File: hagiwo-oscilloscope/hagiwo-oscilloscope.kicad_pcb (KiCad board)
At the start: 2 copper layers, 40.2 x 111.8 mm, 25 parts, among them J1 Encoder Header, J2 10-Pin uZeus Power, J3 OLED Header, J4 Input Header, U1 Opamp_Dual

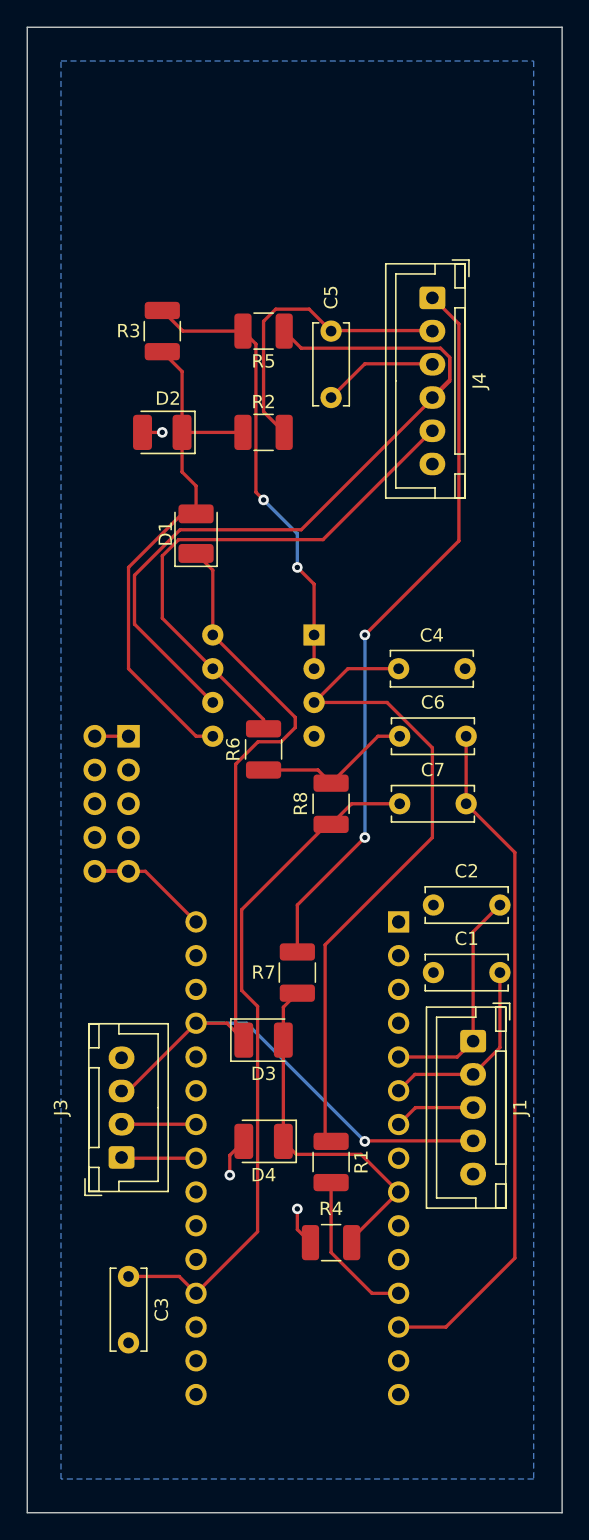
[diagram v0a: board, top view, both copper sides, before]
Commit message: o-scope rev2
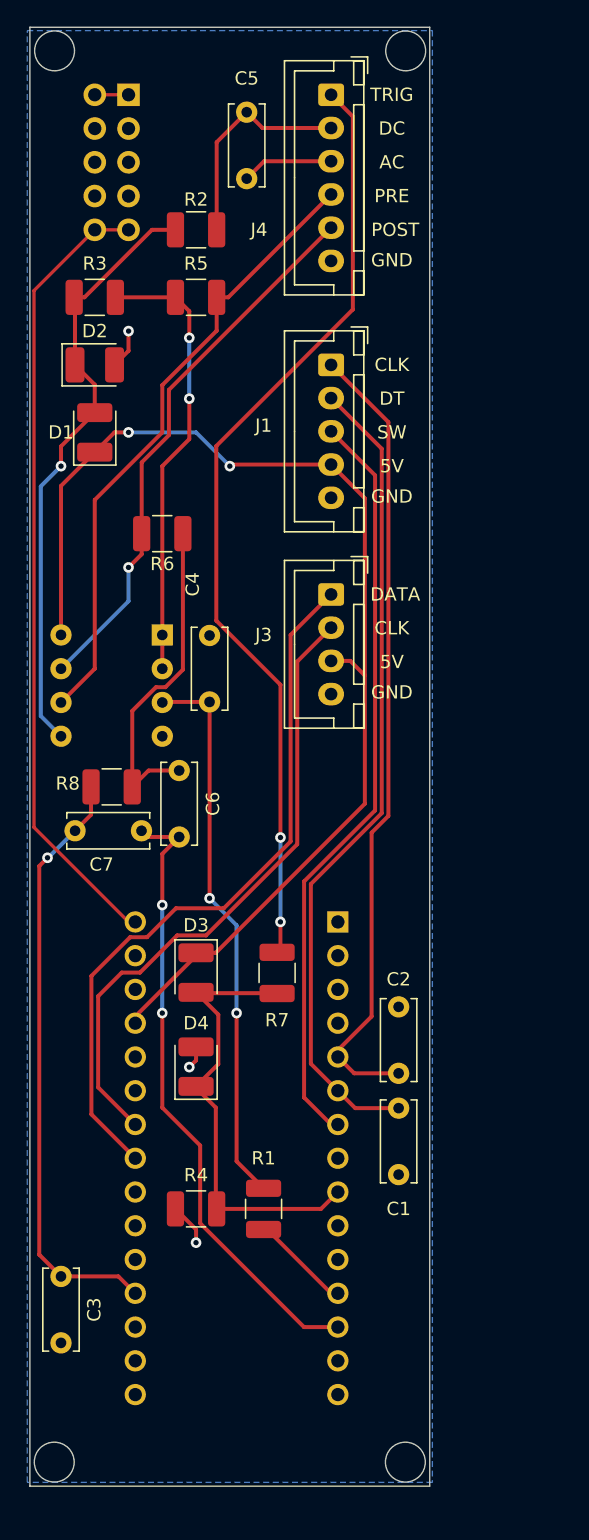
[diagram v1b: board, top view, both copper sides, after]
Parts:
- moved J1 52.0 mm to (66.0, 55.9)
- moved J2 48.3 mm to (50.8, 35.6)
- moved J3 45.2 mm to (66.0, 73.2), turned to -90 degrees
- moved C7 24.5 mm to (51.8, 90.9)
- moved C6 22.9 mm to (54.6, 91.4), turned to 90 degrees
- moved R6 17.9 mm to (53.3, 68.6), turned to 180 degrees
- moved C5 17.7 mm to (59.7, 36.9)
- moved J4 17.1 mm to (66.0, 35.6)
- moved R8 16.6 mm to (49.5, 87.6), turned to 0 degrees
- moved R2 16.1 mm to (55.9, 45.7)
- moved C2 14.8 mm to (71.1, 109.2), turned to 90 degrees
- moved C4 14.4 mm to (56.9, 81.2), turned to 90 degrees
- moved C1 12.7 mm to (71.1, 111.8), turned to -90 degrees
- moved U1 11.4 mm to (53.3, 76.2)
- moved D1 10.8 mm to (48.3, 61.0)
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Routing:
- net EncoderSW: track 6.13 -> 56.6 mm
- net OLEDData: track 5.63 -> 54.1 mm
- net +12V: track 11.7 -> 59.4 mm
- net EncoderDT: track 14.6 -> 61.9 mm
- net EncoderCLK: track 17.2 -> 60.0 mm
- net OLEDClock: track 5.61 -> 47.9 mm
- net TriggerJack: track 55.1 -> 71.2 mm
- net PreGain: track 60.4 -> 47.1 mm
- net Net-(C6-Pad2): track 12.1 -> 25.1 mm
- net Net-(C4-Pad1): track 50.9 -> 41.8 mm, vias 0 -> 2
- net +5V: track 79.2 -> 87.7 mm, vias 1 -> 2
- net SignalIn: track 52.1 -> 45.3 mm, vias 0 -> 1
- net DCInput: track 22.8 -> 16.6 mm
- net ExternalTrigger: track 27.1 -> 32.8 mm
- net Net-(D1-Pad2): track 40.6 -> 45.6 mm, vias 0 -> 1
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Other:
- board size 40.2 x 111.8 mm -> 30.1 x 109.8 mm
- board text added: "5V"
- board text added: "AC"
- board text added: "CLK"
- board text added: "DATA"
- board text added: "DC"
- board text added: "DT"
- board text added: "O-Scope Rev 2 10/3/2022"
- board text added: "POST"
- board text added: "PRE"
- board text added: "SW"
- board text added: "TRIG"
